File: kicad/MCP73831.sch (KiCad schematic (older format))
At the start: 13 parts, among them J1 BATT, U2 MCP73831-2

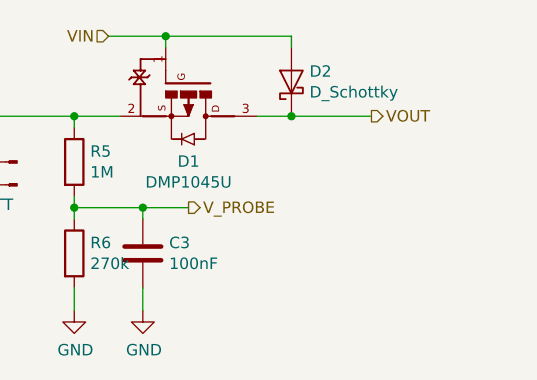
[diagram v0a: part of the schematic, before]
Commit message: first pcb v1.0
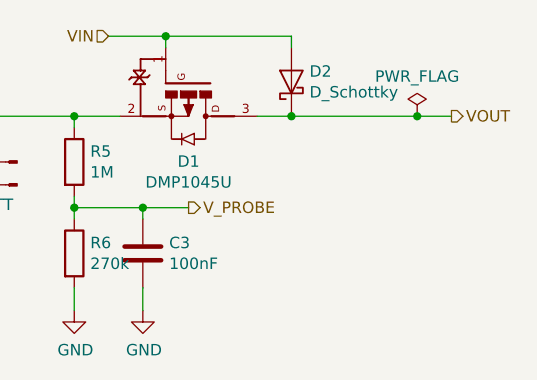
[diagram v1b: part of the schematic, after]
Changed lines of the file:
@@
 Text HLabel 4250 2500 0    50   Input ~ 0
 VIN
-Text HLabel 8850 2700 2    50   Output ~ 0
+Text HLabel 9200 2700 2    50   Output ~ 0
 VOUT
 Wire Wire Line
@@
 Wire Wire Line
 	7550 3450 7550 3550
-Wire Wire Line
-	7850 3450 7850 3550
 Wire Wire Line
 	7850 3150 7850 3100
@@
 Wire Wire Line
 	8350 2700 8500 2700
-Wire Wire Line
-	8850 2700 8500 2700
 Connection ~ 8500 2700
 Wire Wire Line
@@
 Text HLabel 8050 3100 2    50   Output ~ 0
 V_PROBE
+$Comp
+L power:PWR_FLAG #FLG0104
+U 1 1 5C448D6B
+P 9050 2700
+F 0 "#FLG0104" H 9050 2775 50  0001 C CNN
+F 1 "PWR_FLAG" H 9050 2874 50  0000 C CNN
+F 2 "" H 9050 2700 50  0001 C CNN
+F 3 "~" H 9050 2700 50  0001 C CNN
+	1    9050 2700
+	1    0    0    -1
+$EndComp
+Wire Wire Line
+	8500 2700 9050 2700
+Wire Wire Line
+	9050 2700 9200 2700
+Connection ~ 9050 2700
+Wire Wire Line
+	7850 3450 7850 3550
 $EndSCHEMATC
